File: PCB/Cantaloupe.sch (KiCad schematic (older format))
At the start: 123 parts, among them J1 USB_In, J2 OLED, J3 Link, J4 Debug, J5 Trackball, Q1 2N7002, Q2 AO3401A, SW1 MX, SW10 MX, SW11 MX, SW12 MX, SW13 MX, SW14 MX, SW15 MX, SW16 MX, SW17 MX, SW18 MX, SW19 MX, SW2 MX, SW20 MX, SW21 MX, SW22 MX, SW23 MX, SW24 MX, SW25 MX, SW26 MX, SW27 MX, SW28 MX, SW29 MX, SW3 MX, SW30 MX, SW31 Encoder, SW32 MX, SW4 MX, SW5 MX, SW6 MX, SW7 MX, SW8 MX, SW9 MX, U1 STM32F303CCTx, U2 SRV05-4, U3 SRV05-4, U4 XC6206P332MR, U5 LMV321, Y1 8MHz

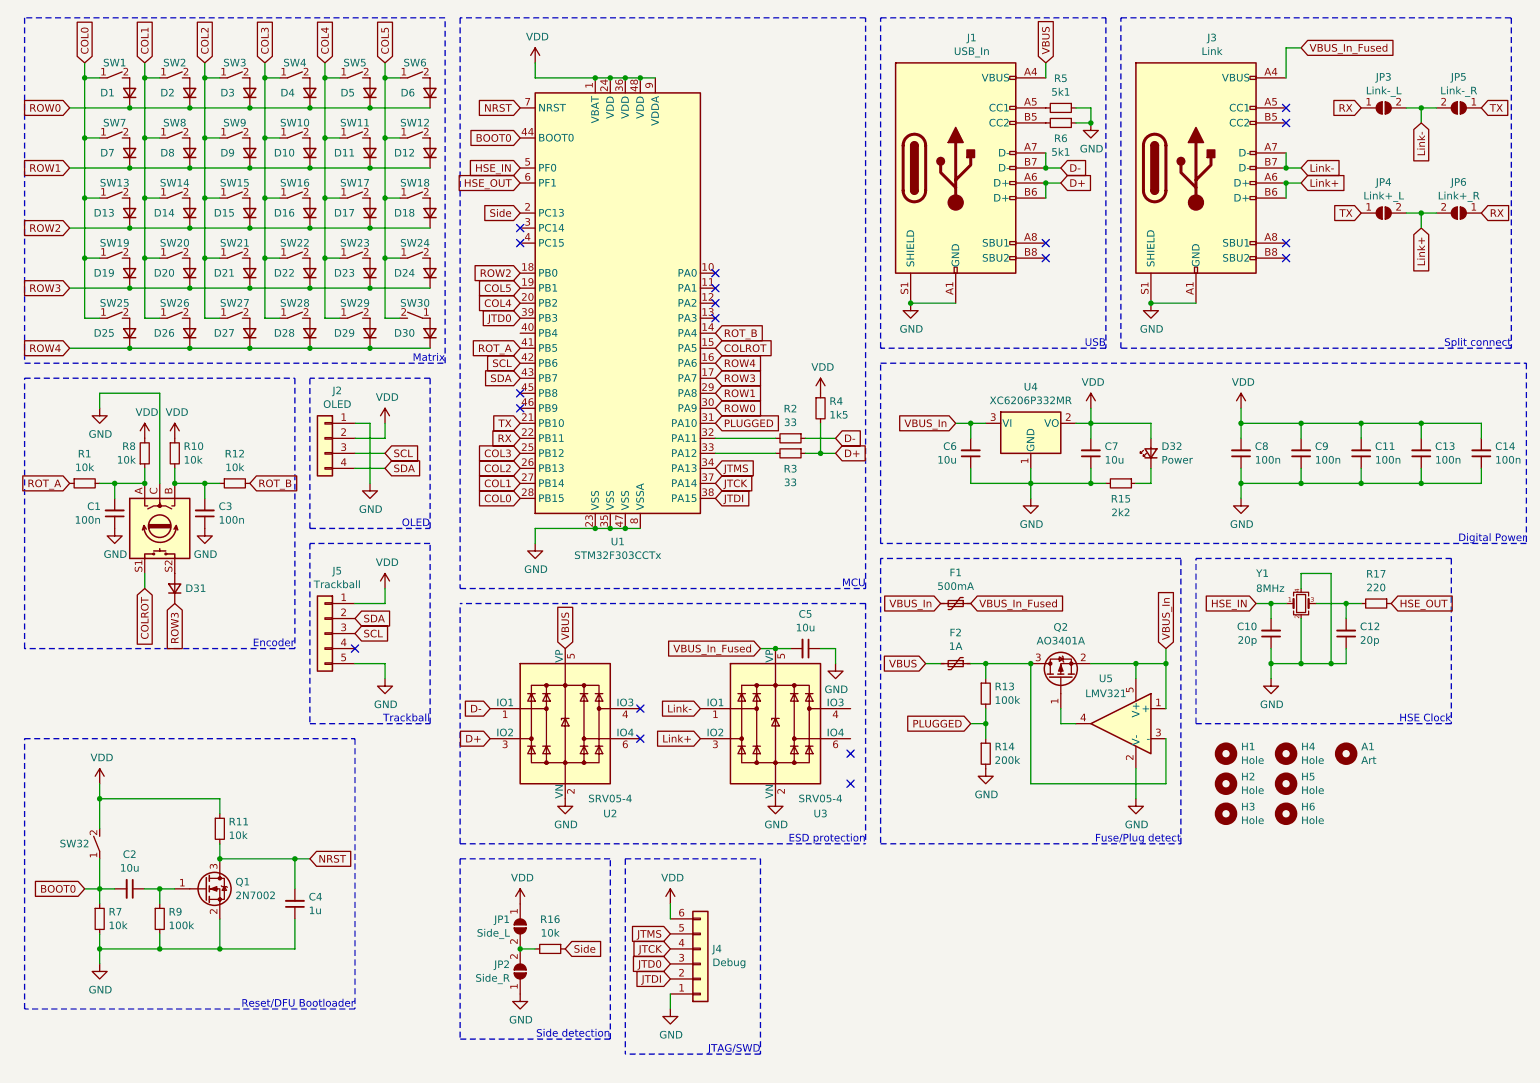
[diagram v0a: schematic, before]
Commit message: STM32F4x0 version
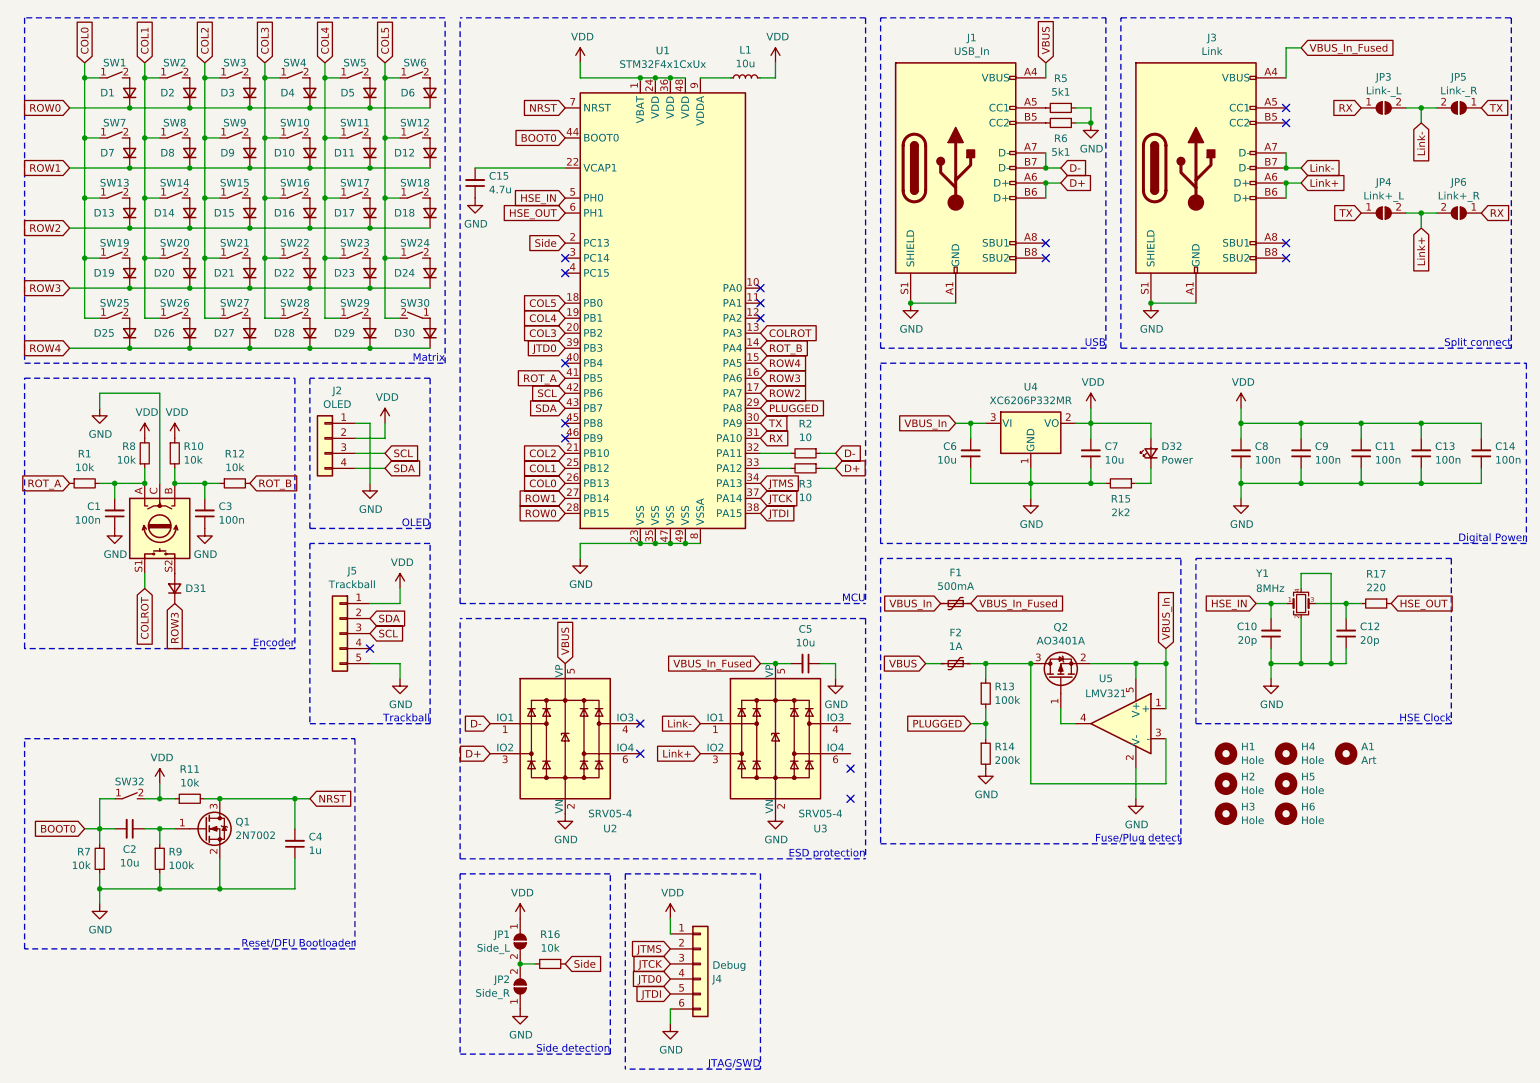
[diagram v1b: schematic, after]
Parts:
- removed R4: 1k5, Resistor_SMD:R_0603_1608Metric, symbol Device:R_Small
- removed U1: STM32F303CCTx, Package_QFP:LQFP-48_7x7mm_P0.5mm, symbol MCU_ST_STM32F3:STM32F303CCTx
- added C15: 4.7u, Capacitor_SMD:C_0603_1608Metric, symbol Device:C_Small
- added L1: 10u, Inductor_SMD:L_0603_1608Metric, symbol Device:L_Small
- added U1: STM32F4x1CxUx, Package_DFN_QFN:QFN-48-1EP_7x7mm_P0.5mm_EP5.6x5.6mm, symbol MCU_ST_STM32F4:STM32F411CCUx
- R2, R3: value 33 -> 10
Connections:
- net BOOT0: now also R7.2, U1.44 (BOOT0); no longer R7.1
- net COL0: now also U1.26 (PB13)
- net COL1: now also U1.25 (PB12)
- net COL2: now also U1.21 (PB10)
- net COL3: now also U1.20 (PB2)
- net COL4: now also U1.19 (PB1)
- net COL5: now also U1.18 (PB0)
- net COLROT: now also U1.13 (PA3)
- net GND: now also J4.6 (Pin_6), R7.1, C15.1, U1.23 (VSS), U1.35 (VSS), U1.47 (VSS), U1.49 (VSS), U1.8 (VSSA); no longer J4.1 (Pin_1), R7.2
- net HSE_IN: now also U1.5 (PH0)
- net HSE_OUT: now also U1.6 (PH1)
- net JTCK: now also J4.3 (Pin_3), U1.37 (PA14); no longer J4.4 (Pin_4)
- net JTD0: now also J4.4 (Pin_4), U1.39 (PB3); no longer J4.3 (Pin_3)
- net JTDI: now also J4.5 (Pin_5), U1.38 (PA15); no longer J4.2 (Pin_2)
- net JTMS: now also J4.2 (Pin_2), U1.34 (PA13); no longer J4.5 (Pin_5)
- net NRST: now also U1.7 (NRST)
- net PLUGGED: now also U1.29 (PA8)
- net ROT_A: now also U1.41 (PB5)
- net ROT_B: now also U1.14 (PA4)
- net ROW0: now also U1.28 (PB15)
- net ROW1: now also U1.27 (PB14)
- net ROW2: now also U1.17 (PA7)
- net ROW3: now also U1.16 (PA6)
- net ROW4: now also U1.15 (PA5)
- net RX: now also U1.31 (PA10)
- net SCL: now also U1.42 (PB6)
- net SDA: now also U1.43 (PB7)
- net Side: now also U1.2 (PC13)
- net TX: now also U1.30 (PA9)
- net VDD: now also J4.1 (Pin_1), L1.2, U1.1 (VBAT), U1.24 (VDD), U1.36 (VDD), U1.48 (VDD); no longer J4.6 (Pin_6)
- net at R2.2: now also U1.32 (PA11)
- net at R3.2: now also U1.33 (PA12)
- new net: C15.2, U1.22 (VCAP1)
- new net: L1.1, U1.9 (VDDA)
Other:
- moved on the sheet: C2, C4, C5, J4, J5, JP1, JP2, Q1, R11, R16, R2, R3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
